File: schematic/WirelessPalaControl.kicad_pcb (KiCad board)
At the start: 2 copper layers, 26.7 x 35.1 mm, 20 parts, among them J1 6P6C, J2 MCU UART, Q1 BC847B, Q2 BC847B, U1 SI8621, U2 WeMos_mini

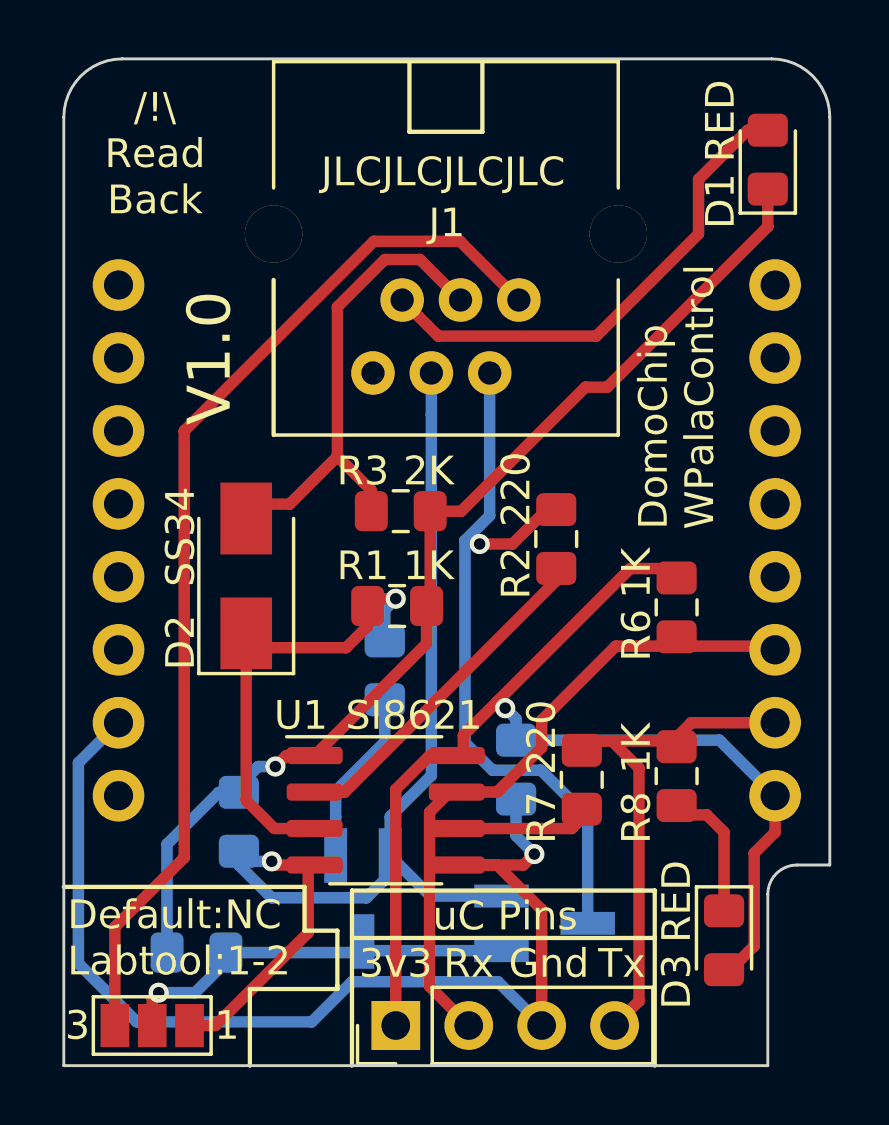
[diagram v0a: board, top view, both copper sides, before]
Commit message: Update PCB fix size V1.1
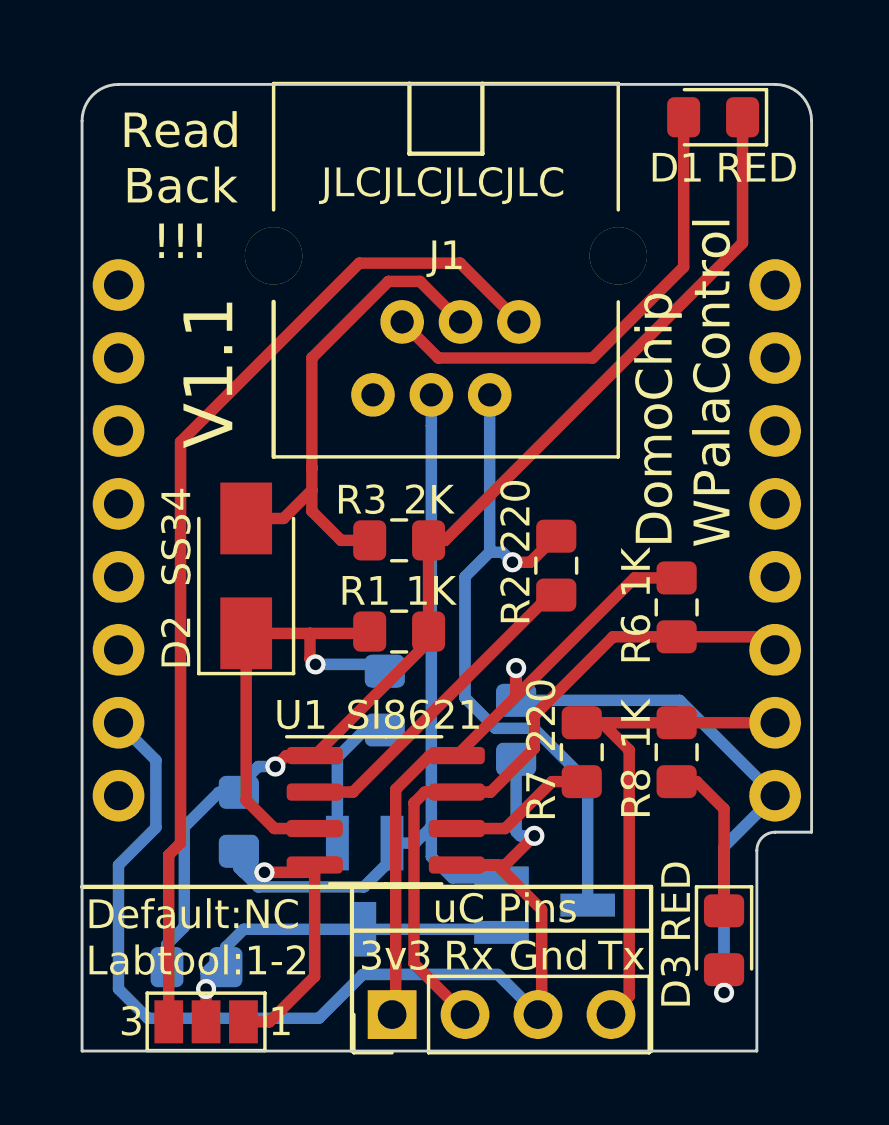
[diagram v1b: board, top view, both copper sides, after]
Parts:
- moved D1 2.41 mm to (45.5, 25.9), turned to 180 degrees
- moved JP1 1.88 mm to (27.8, 57.4)
- moved C2 1.39 mm to (38.6, 47.2)
- moved R4 1.05 mm to (34.0, 46.2)
- moved R3 1.02 mm to (34.5, 40.6)
- moved R7 0.96 mm to (40.9, 48.0)
- moved R2 0.93 mm to (40.0, 41.5)
- moved R1 0.89 mm to (34.5, 43.8)
- moved R8 0.83 mm to (44.2, 48.0)
- moved J1 0.76 mm to (36.2, 30.7)
- moved Q2 0.63 mm to (39.6, 53.3)
- moved R5 0.51 mm to (27.5, 55.5)
- moved Q1 0.43 mm to (33.3, 52.7)
- moved J2 0.40 mm to (34.3, 57.1)
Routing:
- net /VDD2: track 39.9 -> 42.3 mm, vias 1 -> 2
- net /Tx-RxH: track 25.8 -> 23.5 mm
- net /VDD1: track 37.2 -> 39.1 mm
- net /GND1: track 38.8 -> 37.4 mm
- net Net-(J1-Pad6): track 36.9 -> 35.6 mm
- net Net-(D3-Pad1): track 4.31 -> 5.59 mm
- net /GND2: track 39.1 -> 40.3 mm
- net /RXuC: track 23.0 -> 23.9 mm
- net Net-(Q1-Pad1): track 5.80 -> 5.03 mm
- net Net-(R7-Pad2): track 4.27 -> 5.03 mm
- net /Q2B: track 14.0 -> 13.3 mm
- net Net-(R2-Pad2): track 11.8 -> 11.3 mm
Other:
- board size 26.7 x 35.1 mm -> 25.4 x 33.7 mm
- board text added: "!!!"
- board text added: "DomoChip WPalaControl V1.1"
- board text added: "Read Back !!!"
- board text added: "Use RJ11 cross cable (phone standard)"
- board text added: "V1.1"
- board text removed: "/!\ Read Back"
- board text removed: "/!\ Use RJ11 cross cable (phone standard) /!\"
- board text removed: "DomoChip WPalaControl V1.0"
- board text removed: "V1.0"
